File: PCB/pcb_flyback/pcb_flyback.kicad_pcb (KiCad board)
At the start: 2 copper layers, 31 parts, among them Q1 IRF540N, U1 TL494, U2 PC817

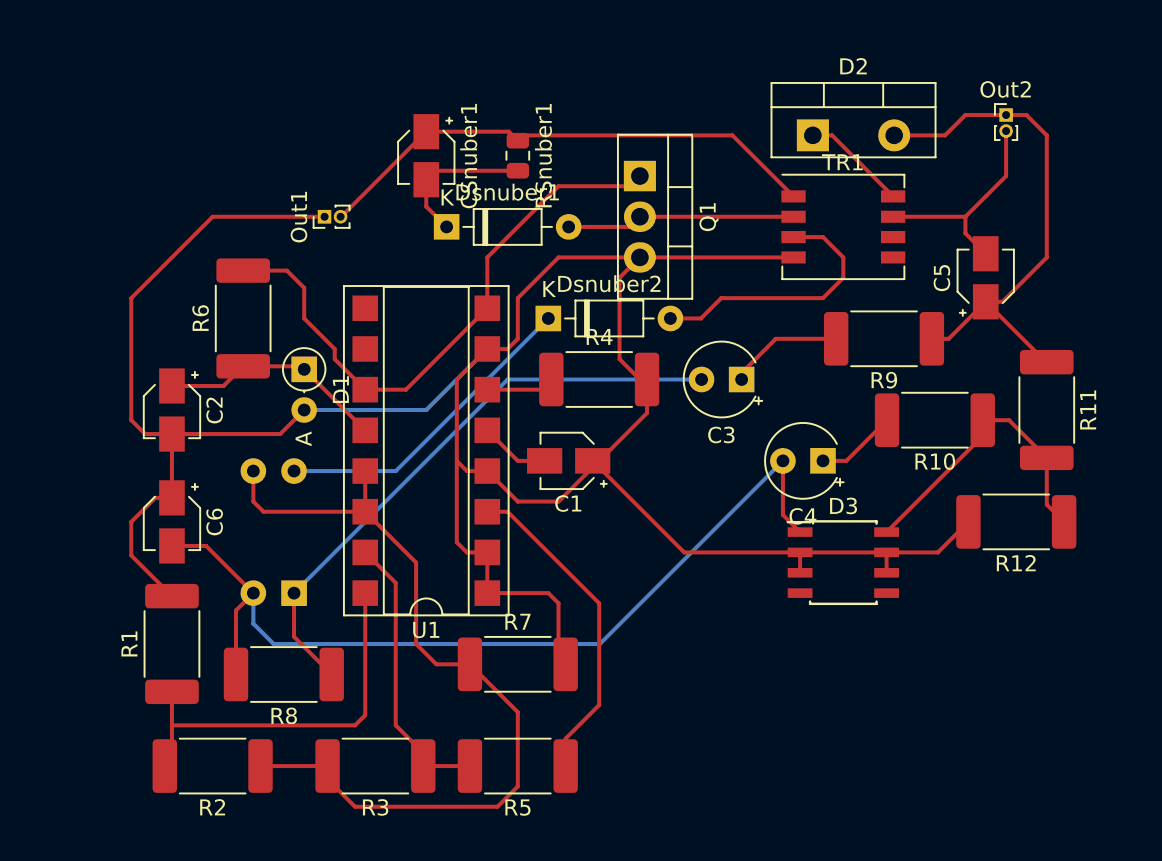
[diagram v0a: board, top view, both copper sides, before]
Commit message: cambios en PCB
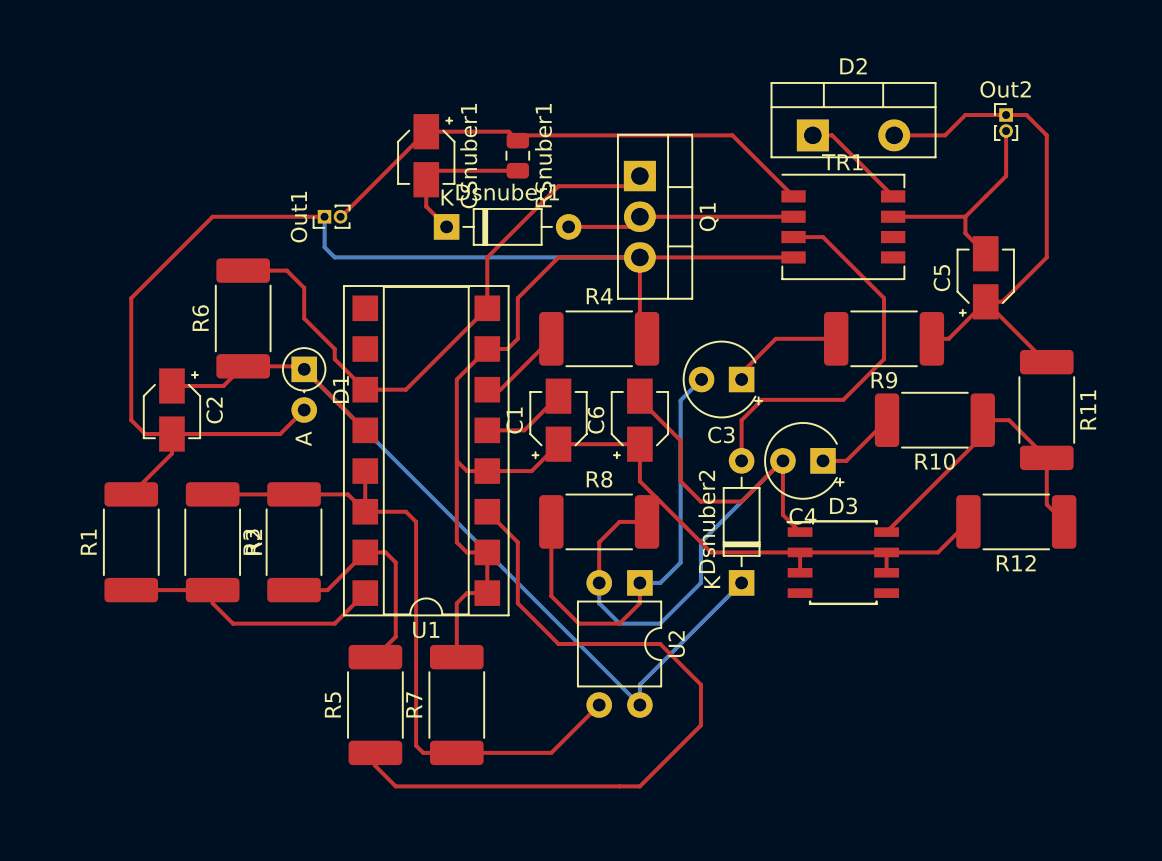
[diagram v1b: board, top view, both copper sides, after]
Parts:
- U2: moved to F.Cu
- moved C6 29.9 mm to (116.8, 106.7), turned to 90 degrees
- moved R8 21.9 mm to (114.3, 113.0), turned to 0 degrees
- moved U2 21.6 mm to (116.8, 116.8), turned to 270 degrees
- moved Dsnuber2 20.4 mm to (123.2, 116.8), turned to 90 degrees
- moved R3 14.9 mm to (95.2, 114.3), turned to 90 degrees
- moved R2 14.0 mm to (90.2, 114.3), turned to 270 degrees
- moved R5 9.67 mm to (100.3, 124.5), turned to 90 degrees
- moved R1 6.84 mm to (85.1, 114.3)
- moved R7 4.58 mm to (105.4, 124.5), turned to 90 degrees
- moved C1 2.62 mm to (111.8, 106.7), turned to 90 degrees
- moved R4 2.54 mm to (114.3, 101.6)
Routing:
- net Net-(R5-Pad1): track 20.4 -> 45.8 mm
- net Net-(C2-Pad1): track 34.0 -> 54.1 mm
- net Net-(C4-Pad2): track 56.9 -> 44.2 mm
- net GND: track 163.6 -> 151.9 mm
- net Net-(R2-Pad1): track 52.1 -> 42.8 mm
- net Net-(C3-Pad2): track 37.0 -> 27.7 mm
- net Net-(R1-Pad1): track 24.8 -> 16.7 mm
- net Net-(Dsnuber2-Pad2): track 16.8 -> 24.0 mm
- net Net-(R3-Pad1): track 17.8 -> 14.6 mm
- net Net-(R4-Pad1): track 4.26 -> 5.31 mm
- net Net-(C1-Pad2): track 4.37 -> 5.33 mm

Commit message: cambios en los bancos de prueba de fuente y controlador
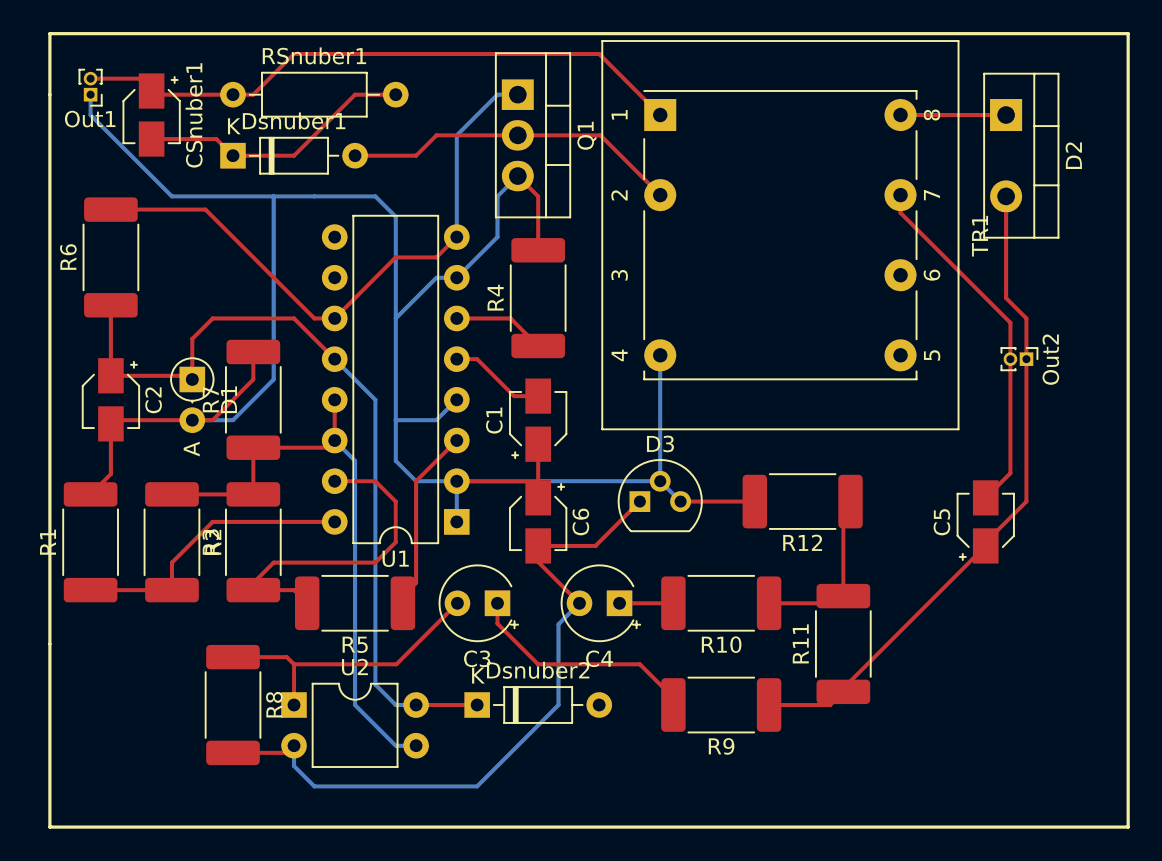
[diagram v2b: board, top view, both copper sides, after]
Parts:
- D3: footprint Package_SO:SOIC-8_3.9x4.9mm_P1.27mm -> Package_TO_SOT_THT:TO-92
- RSnuber1: footprint Resistor_SMD:R_0805_2012Metric -> Resistor_THT:R_Axial_DIN0207_L6.3mm_D2.5mm_P10.16mm_Horizontal
- TR1: footprint Transformer_SMD:Pulse_PA2777NL -> Transformer_THT:Transformer_Breve_TEZ-22x24
- U1: footprint Package_DIP:DIP-16_W7.62mm_SMDSocket_SmallPads -> Package_DIP:DIP-16_W7.62mm
- moved R8 25.6 mm to (91.4, 124.5), turned to 270 degrees
- moved R9 25.0 mm to (121.9, 124.5)
- moved R7 22.9 mm to (92.7, 105.4)
- moved U2 22.9 mm to (95.2, 124.5), turned to 0 degrees
- moved C3 20.7 mm to (108.0, 118.1)
- moved R11 19.4 mm to (129.5, 120.7), turned to 90 degrees
- moved RSnuber1 18.2 mm to (91.4, 86.4), turned to 0 degrees
- moved Dsnuber2 18.2 mm to (106.7, 124.5), turned to 0 degrees
- moved R10 17.6 mm to (121.9, 118.1)
- moved CSnuber1 17.3 mm to (86.4, 87.6)
- moved Out1 16.5 mm to (82.5, 86.4), turned to 180 degrees
- moved C4 15.5 mm to (115.6, 118.1)
- moved Out2 15.3 mm to (141.0, 102.9), turned to 270 degrees
- moved C5 15.2 mm to (138.4, 113.0)
- moved Dsnuber1 14.1 mm to (91.4, 90.2)
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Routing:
- net Net-(R5-Pad1): track 45.8 -> 11.6 mm
- net Net-(Dsnuber2-Pad2): track 24.0 -> 0.00 mm
- net GND: track 151.9 -> 138.1 mm
- net Net-(C3-Pad2): track 27.7 -> 18.3 mm
- net Net-(C5-Pad2): track 13.7 -> 22.4 mm
- net Net-(C5-Pad1): track 32.8 -> 41.2 mm
- net Net-(C3-Pad1): track 6.56 -> 14.6 mm
- net Net-(D3-Pad8): track 18.9 -> 10.9 mm
- net Net-(CSnuber1-Pad2): track 9.42 -> 17.2 mm
- net Net-(Dsnuber1-Pad2): track 14.3 -> 21.1 mm
- net Net-(CSnuber1-Pad1): track 32.1 -> 38.6 mm
- net Net-(R3-Pad1): track 14.6 -> 21.0 mm
- net Net-(R2-Pad1): track 42.8 -> 37.7 mm
- net Net-(C2-Pad1): track 54.1 -> 50.8 mm
- net Net-(C4-Pad1): track 5.05 -> 3.36 mm
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- added copper zone on B.Cu, net GND
